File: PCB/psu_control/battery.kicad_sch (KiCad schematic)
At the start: 5 parts

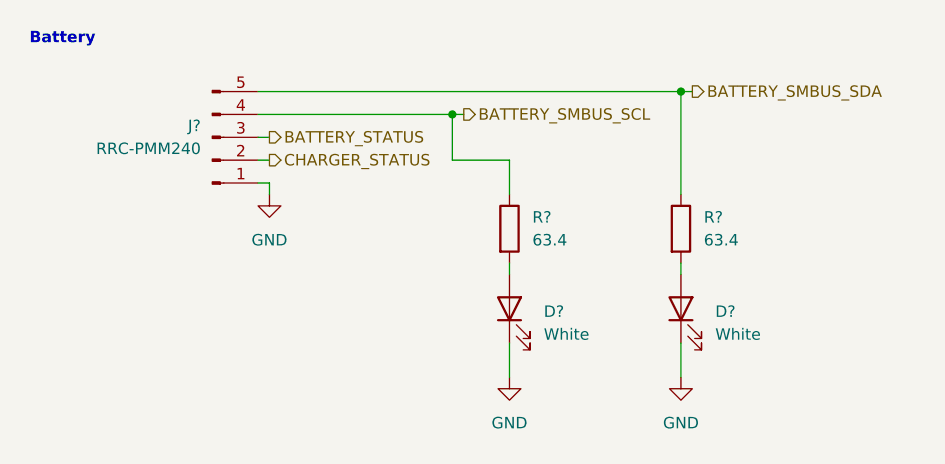
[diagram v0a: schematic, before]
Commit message: psu_control v4 is completed
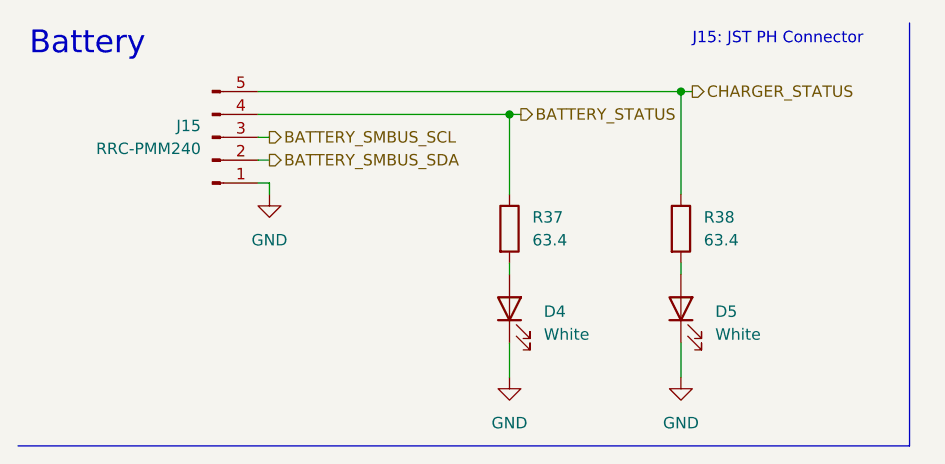
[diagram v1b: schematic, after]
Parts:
- D4, D5: renamed from D?; footprint (none) -> Connector_JST:JST_PH_B2B-PH-K_1x02_P2.00mm_Vertical
- J15: renamed from J?; footprint (none) -> Connector_JST:JST_PH_B5B-PH-K_1x05_P2.00mm_Vertical
- R37, R38: renamed from R?; footprint (none) -> Resistor_SMD:R_0805_2012Metric
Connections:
- net BATTERY_SMBUS_SCL: now also J15.3 (Pin_3); no longer J15.4 (Pin_4), R37.1
- net BATTERY_SMBUS_SDA: now also J15.2 (Pin_2); no longer J15.5 (Pin_5), R38.1
- net BATTERY_STATUS: now also J15.4 (Pin_4), R37.1; no longer J15.3 (Pin_3)
- net CHARGER_STATUS: now also J15.5 (Pin_5), R38.1; no longer J15.2 (Pin_2)
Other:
- note added: "J15: JST PH Connector"
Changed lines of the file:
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@@
 (kicad_sch (version 20211123) (generator eeschema)
   (paper "A4")
+  (junction (at 67.31 22.86) (diameter 0) (color 0 0 0 0)
+  )
   (junction (at 86.36 20.32) (diameter 0) (color 0 0 0 0)
-  )
-  (junction (at 60.96 22.86) (diameter 0) (color 0 0 0 0)
-  )
-  (wire (pts (xy 39.37 22.86) (xy 60.96 22.86))
-    (stroke (width 0) (type default) (color 0 0 0 0))
   )
   (wire (pts (xy 86.36 48.26) (xy 86.36 52.07))
     (stroke (width 0) (type default) (color 0 0 0 0))
   )
-  (wire (pts (xy 86.36 20.32) (xy 87.63 20.32))
+  (wire (pts (xy 67.31 22.86) (xy 68.58 22.86))
+    (stroke (width 0) (type default) (color 0 0 0 0))
+  )
+  (wire (pts (xy 86.36 20.32) (xy 86.36 31.75))
+    (stroke (width 0) (type default) (color 0 0 0 0))
+  )
+  (wire (pts (xy 39.37 22.86) (xy 67.31 22.86))
     (stroke (width 0) (type default) (color 0 0 0 0))
   )
@@
     (stroke (width 0) (type default) (color 0 0 0 0))
   )
-  (wire (pts (xy 60.96 22.86) (xy 62.23 22.86))
-    (stroke (width 0) (type default) (color 0 0 0 0))
-  )
   (wire (pts (xy 39.37 27.94) (xy 40.64 27.94))
     (stroke (width 0) (type default) (color 0 0 0 0))
   )
-  (wire (pts (xy 60.96 27.94) (xy 67.31 27.94))
+  (polyline (pts (xy 111.76 12.7) (xy 111.76 59.69))
     (stroke (width 0) (type default) (color 0 0 0 0))
   )
   (wire (pts (xy 39.37 25.4) (xy 40.64 25.4))
-    (stroke (width 0) (type default) (color 0 0 0 0))
-  )
-  (wire (pts (xy 86.36 20.32) (xy 86.36 31.75))
-    (stroke (width 0) (type default) (color 0 0 0 0))
-  )
-  (wire (pts (xy 67.31 27.94) (xy 67.31 31.75))
     (stroke (width 0) (type default) (color 0 0 0 0))
   )
@@
     (stroke (width 0) (type default) (color 0 0 0 0))
   )
+  (wire (pts (xy 86.36 20.32) (xy 87.63 20.32))
+    (stroke (width 0) (type default) (color 0 0 0 0))
+  )
+  (polyline (pts (xy 12.7 59.69) (xy 111.76 59.69))
+    (stroke (width 0) (type default) (color 0 0 0 0))
+  )
   (wire (pts (xy 40.64 30.48) (xy 40.64 31.75))
     (stroke (width 0) (type default) (color 0 0 0 0))
   )
-  (wire (pts (xy 60.96 22.86) (xy 60.96 27.94))
+  (wire (pts (xy 67.31 22.86) (xy 67.31 31.75))
     (stroke (width 0) (type default) (color 0 0 0 0))
   )
-  (text "Battery" (at 13.97 15.24 0)
-    (effects (font (size 1.27 1.27) bold) (justify left bottom))
+  (text "Battery" (at 13.97 16.51 0)
+    (effects (font (size 2.54 2.54)) (justify left bottom))
   )
-  (hierarchical_label "BATTERY_STATUS" (shape output) (at 40.64 25.4 0)
+  (text "J15: JST PH Connector" (at 87.63 15.24 0)
+    (effects (font (size 1.27 1.27)) (justify left bottom))
+  )
+  (hierarchical_label "BATTERY_STATUS" (shape output) (at 68.58 22.86 0)
     (effects (font (size 1.27 1.27)) (justify left))
   )
-  (hierarchical_label "BATTERY_SMBUS_SDA" (shape output) (at 87.63 20.32 0)
+  (hierarchical_label "BATTERY_SMBUS_SDA" (shape output) (at 40.64 27.94 0)
     (effects (font (size 1.27 1.27)) (justify left))
   )
-  (hierarchical_label "BATTERY_SMBUS_SCL" (shape output) (at 62.23 22.86 0)
+  (hierarchical_label "BATTERY_SMBUS_SCL" (shape output) (at 40.64 25.4 0)
     (effects (font (size 1.27 1.27)) (justify left))
   )
-  (hierarchical_label "CHARGER_STATUS" (shape output) (at 40.64 27.94 0)
+  (hierarchical_label "CHARGER_STATUS" (shape output) (at 87.63 20.32 0)
     (effects (font (size 1.27 1.27)) (justify left))
   )
   (symbol (lib_id "Device:R") (at 67.31 35.56 0) (unit 1)
     (in_bom yes) (on_board yes) (fields_autoplaced)
-    (property "Reference" "R?" (id 0) (at 69.85 34.2899 0)
+    (property "Reference" "R37" (id 0) (at 69.85 34.2899 0)
       (effects (font (size 1.27 1.27)) (justify left))
     )
@@
       (effects (font (size 1.27 1.27)) (justify left))
     )
-    (property "Footprint" "" (id 2) (at 65.532 35.56 90)
+    (property "Footprint" "Resistor_SMD:R_0805_2012Metric" (id 2) (at 65.532 35.56 90)
       (effects (font (size 1.27 1.27)) hide)
     )
@@
   (symbol (lib_id "Device:R") (at 86.36 35.56 0) (unit 1)
     (in_bom yes) (on_board yes) (fields_autoplaced)
-    (property "Reference" "R?" (id 0) (at 88.9 34.2899 0)
+    (property "Reference" "R38" (id 0) (at 88.9 34.2899 0)
       (effects (font (size 1.27 1.27)) (justify left))
     )
@@
       (effects (font (size 1.27 1.27)) (justify left))
     )
-    (property "Footprint" "" (id 2) (at 84.582 35.56 90)
+    (property "Footprint" "Resistor_SMD:R_0805_2012Metric" (id 2) (at 84.582 35.56 90)
       (effects (font (size 1.27 1.27)) hide)
     )
@@
   (symbol (lib_id "Device:LED") (at 67.31 44.45 90) (unit 1)
     (in_bom yes) (on_board yes) (fields_autoplaced)
-    (property "Reference" "D?" (id 0) (at 71.12 44.7674 90)
+    (property "Reference" "D4" (id 0) (at 71.12 44.7674 90)
       (effects (font (size 1.27 1.27)) (justify right))
     )
@@
       (effects (font (size 1.27 1.27)) (justify right))
     )
-    (property "Footprint" "" (id 2) (at 67.31 44.45 0)
+    (property "Footprint" "Connector_JST:JST_PH_B2B-PH-K_1x02_P2.00mm_Vertical" (id 2) (at 67.31 44.45 0)
       (effects (font (size 1.27 1.27)) hide)
     )
@@
   (symbol (lib_id "Device:LED") (at 86.36 44.45 90) (unit 1)
     (in_bom yes) (on_board yes) (fields_autoplaced)
-    (property "Reference" "D?" (id 0) (at 90.17 44.7674 90)
+    (property "Reference" "D5" (id 0) (at 90.17 44.7674 90)
       (effects (font (size 1.27 1.27)) (justify right))
     )
@@
       (effects (font (size 1.27 1.27)) (justify right))
     )
-    (property "Footprint" "" (id 2) (at 86.36 44.45 0)
+    (property "Footprint" "Connector_JST:JST_PH_B2B-PH-K_1x02_P2.00mm_Vertical" (id 2) (at 86.36 44.45 0)
       (effects (font (size 1.27 1.27)) hide)
     )
@@
   (symbol (lib_id "power:GND") (at 40.64 31.75 0) (unit 1)
     (in_bom yes) (on_board yes) (fields_autoplaced)
-    (property "Reference" "#PWR?" (id 0) (at 40.64 38.1 0)
+    (property "Reference" "#PWR0179" (id 0) (at 40.64 38.1 0)
       (effects (font (size 1.27 1.27)) hide)
     )
@@
   (symbol (lib_id "Connector:Conn_01x05_Male") (at 34.29 25.4 0) (mirror x) (unit 1)
     (in_bom yes) (on_board yes) (fields_autoplaced)
-    (property "Reference" "J?" (id 0) (at 33.02 24.1299 0)
+    (property "Reference" "J15" (id 0) (at 33.02 24.1299 0)
       (effects (font (size 1.27 1.27)) (justify right))
     )
@@
       (effects (font (size 1.27 1.27)) (justify right))
     )
-    (property "Footprint" "" (id 2) (at 34.29 25.4 0)
+    (property "Footprint" "Connector_JST:JST_PH_B5B-PH-K_1x05_P2.00mm_Vertical" (id 2) (at 34.29 25.4 0)
       (effects (font (size 1.27 1.27)) hide)
     )
@@
   (symbol (lib_id "power:GND") (at 67.31 52.07 0) (unit 1)
     (in_bom yes) (on_board yes) (fields_autoplaced)
-    (property "Reference" "#PWR?" (id 0) (at 67.31 58.42 0)
+    (property "Reference" "#PWR0177" (id 0) (at 67.31 58.42 0)
       (effects (font (size 1.27 1.27)) hide)
     )
@@
   (symbol (lib_id "power:GND") (at 86.36 52.07 0) (unit 1)
     (in_bom yes) (on_board yes) (fields_autoplaced)
-    (property "Reference" "#PWR?" (id 0) (at 86.36 58.42 0)
+    (property "Reference" "#PWR0178" (id 0) (at 86.36 58.42 0)
       (effects (font (size 1.27 1.27)) hide)
     )
